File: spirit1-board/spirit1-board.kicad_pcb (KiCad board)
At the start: 2 copper layers, 15 parts, among them CN2 ANT, U1 SPIRIT1, U2 BALF-SPI-02D3, X1 50Mhz

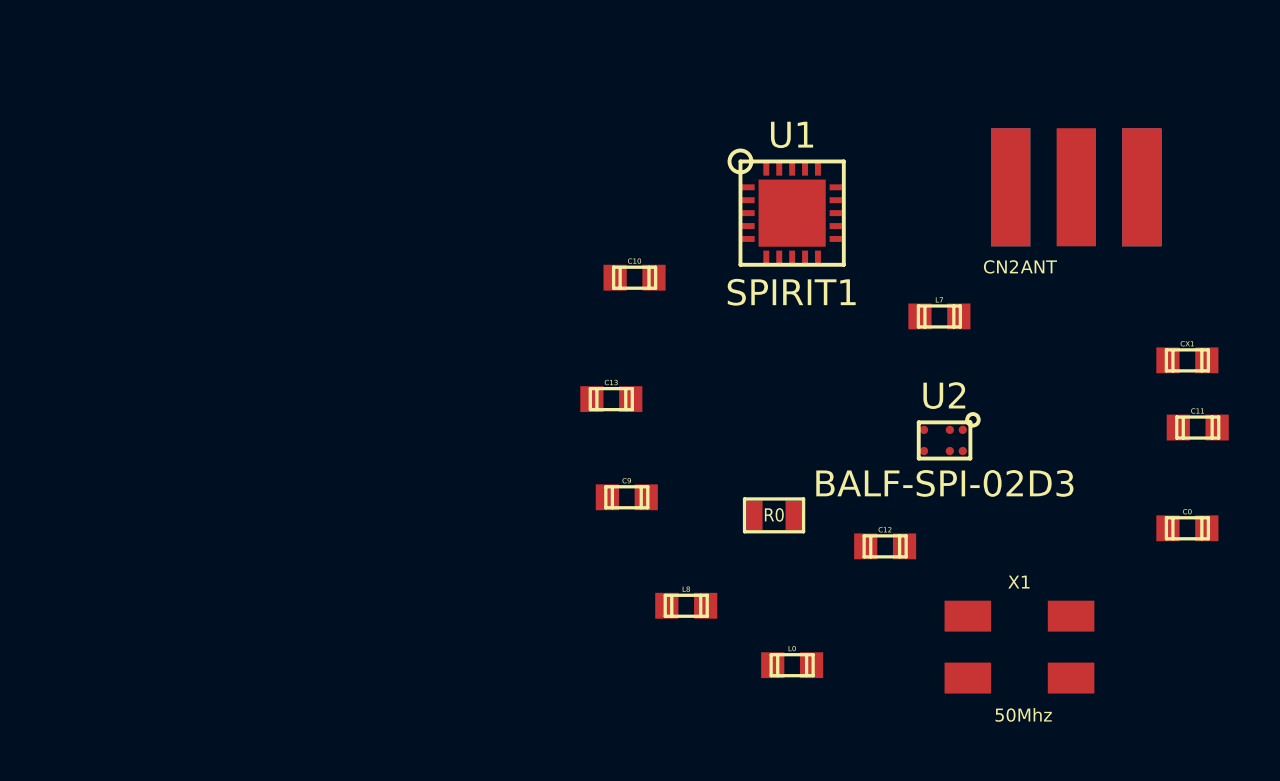
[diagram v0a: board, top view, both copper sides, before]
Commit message: spirit1: Finalise schema and pcb
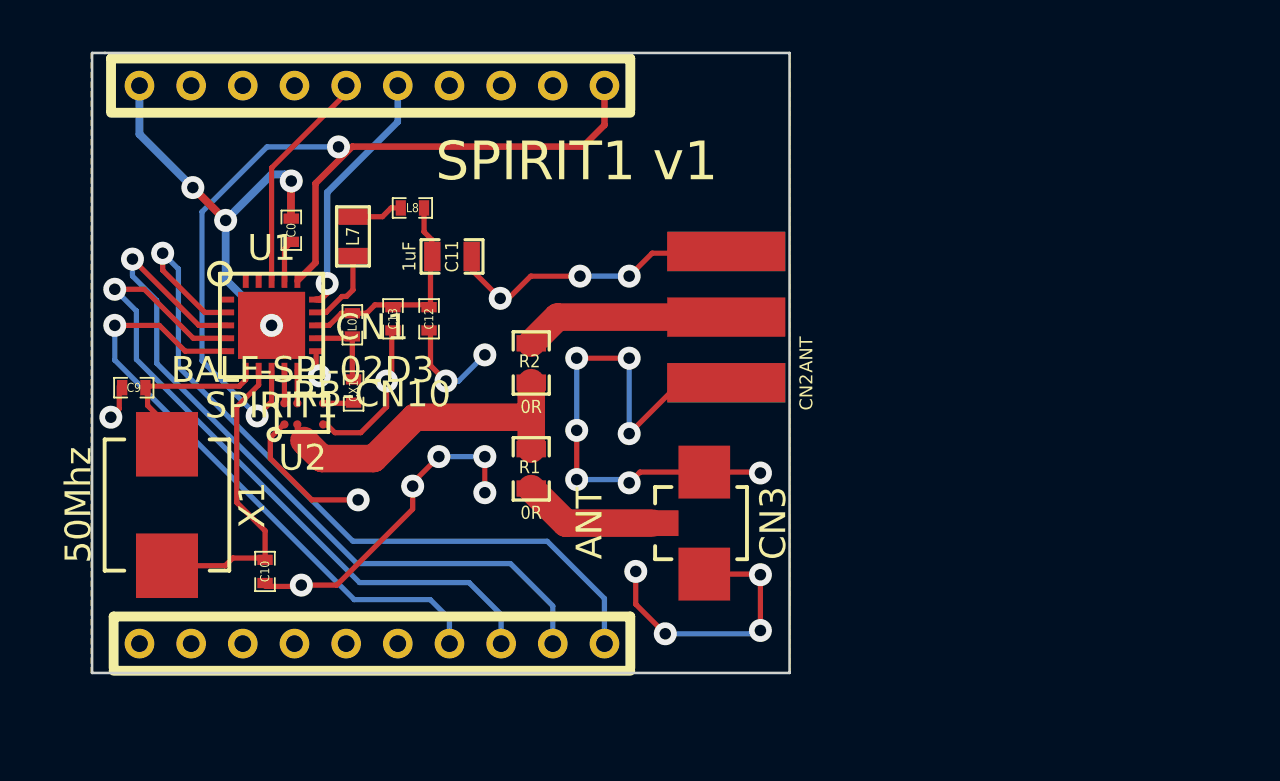
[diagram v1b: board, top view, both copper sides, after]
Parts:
- removed R0: R, SM0603
- added ?: , LOGO_SNOWCAP_BACK, B.Cu at (110.9, 105.5)
- added CN1: RB-CN10, RB_CN10_2mm, F.Cu at (103.8, 107.3)
- added CN3: ANT, U.FL-R-SMT_01, F.Cu at (116.7, 113.7)
- added R1: 0R, SM0603_Resistor, F.Cu at (110.0, 111.6)
- added R2: 0R, SM0603_Resistor, F.Cu at (110.0, 107.5)
- C0, C10, C12, C13, C9, CX1: footprint c_0603 -> SM0402_c
- C11: footprint c_0603 -> SM0603_Capa
- L0, L8: footprint c_0603 -> SM0402
- L7: footprint c_0603 -> SM0603
- X1: footprint CRYSTAL-ABM3B -> CRYSTAL-ABM3-50.000MHZ-D2Y-F-T
- moved C0 36.6 mm to (100.7, 102.4), turned to 90 degrees
- moved X1 33.5 mm to (95.9, 113.0), turned to 270 degrees
- moved CX1 32.3 mm to (103.1, 108.6), turned to 270 degrees
- moved C11 29.6 mm to (106.9, 103.4)
- moved U2 24.9 mm to (101.2, 109.5), turned to 180 degrees
- moved L7 22.9 mm to (103.1, 102.6), turned to 90 degrees
- moved L0 21.5 mm to (103.1, 106.0), turned to 90 degrees
- moved U1 20.6 mm to (99.9, 106.0)
- moved C12 19.7 mm to (106.0, 105.8), turned to 270 degrees
- moved C9 19.6 mm to (94.6, 108.5), turned to 180 degrees
- moved L8 18.7 mm to (105.4, 101.5)
- moved C10 18.3 mm to (99.7, 115.6), turned to 270 degrees
- moved CN2 11.6 mm to (119.8, 105.7), turned to 90 degrees
- moved C13 9.01 mm to (104.6, 105.8), turned to 270 degrees
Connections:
- CN2 pad 1: N-0000033 (its old number) -> N-0000022
- U1 pad 11: N-0000026 -> GND
- U2 pad B1: N-0000033 (its old number) -> N-0000023
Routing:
- net GND: track 0.00 -> 90.7 mm, vias 0 -> 29
- net VCC: track 0.00 -> 35.4 mm, vias 0 -> 2
- net N-0000014: track 0.00 -> 30.4 mm, vias 0 -> 1
- net N-0000015: track 0.00 -> 29.8 mm, vias 0 -> 1
- net N-0000017: track 0.00 -> 27.5 mm, vias 0 -> 1
- net N-0000027: track 0.00 -> 24.2 mm, vias 0 -> 1
- net N-0000023: track 0.00 -> 13.2 mm
- net N-0000033: track 0.00 -> 12.0 mm
- net N-000008: track 0.00 -> 9.68 mm, vias 0 -> 1
- net N-000009: track 0.00 -> 8.75 mm
- net N-0000035: track 0.00 -> 8.65 mm
- net N-0000022: track 0.00 -> 7.97 mm
- net N-0000032: track 0.00 -> 6.85 mm
- net N-0000021: track 0.00 -> 5.23 mm
- net N-0000036: track 0.00 -> 3.10 mm
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- added copper zone on B.Cu, net GND
- added copper zone on F.Cu, net GND
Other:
- board outline added: 27 x 24 mm
- net class 50ohm added: clearance 0.2032, trace_width 1.0668, via_dia 0.889, via_drill 0.635
- net class Default: clearance 0.254 -> 0.2032; trace_width 0.254 -> 0.2032
- rule trace_clearance: 0.254 -> 0.2032
- rule trace_min: 0.254 -> 0.2032
- board text added: "SPIRIT1 v1"
